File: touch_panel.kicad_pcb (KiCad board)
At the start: 2 copper layers, 50 x 50 mm, 46 parts, among them J1 2x4 SMD 2.0 MM, J2 2x4 Regular, Q1 MMBT2222, Q2 MMBT2222, Q3 MMBT2222, Q4 MMBT2222, Q5 MMBT2222, Q6 MMBT2222, SW1 Reset Switch, U1 TTP223_1, U2 TTP223_2, U3 TTP223_3, U4 ESP-12E

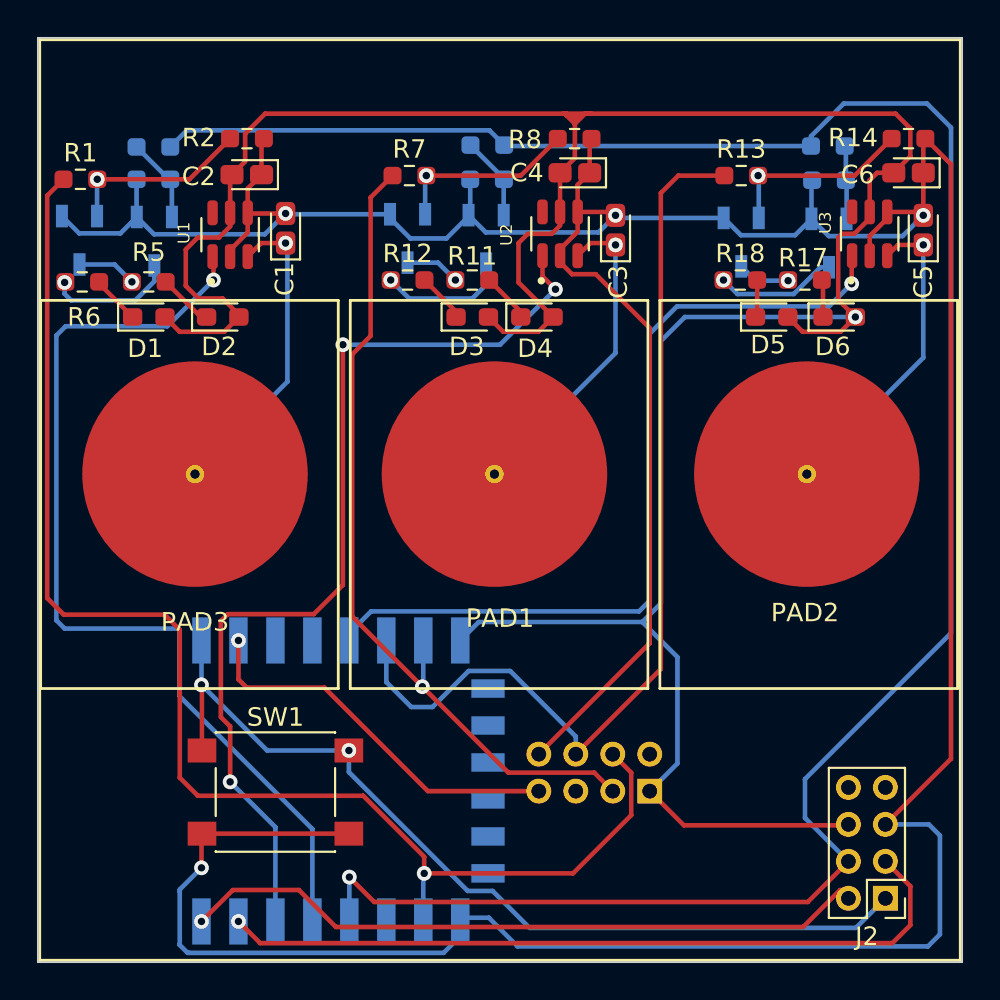
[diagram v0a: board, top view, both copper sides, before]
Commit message: Board finalized for printing
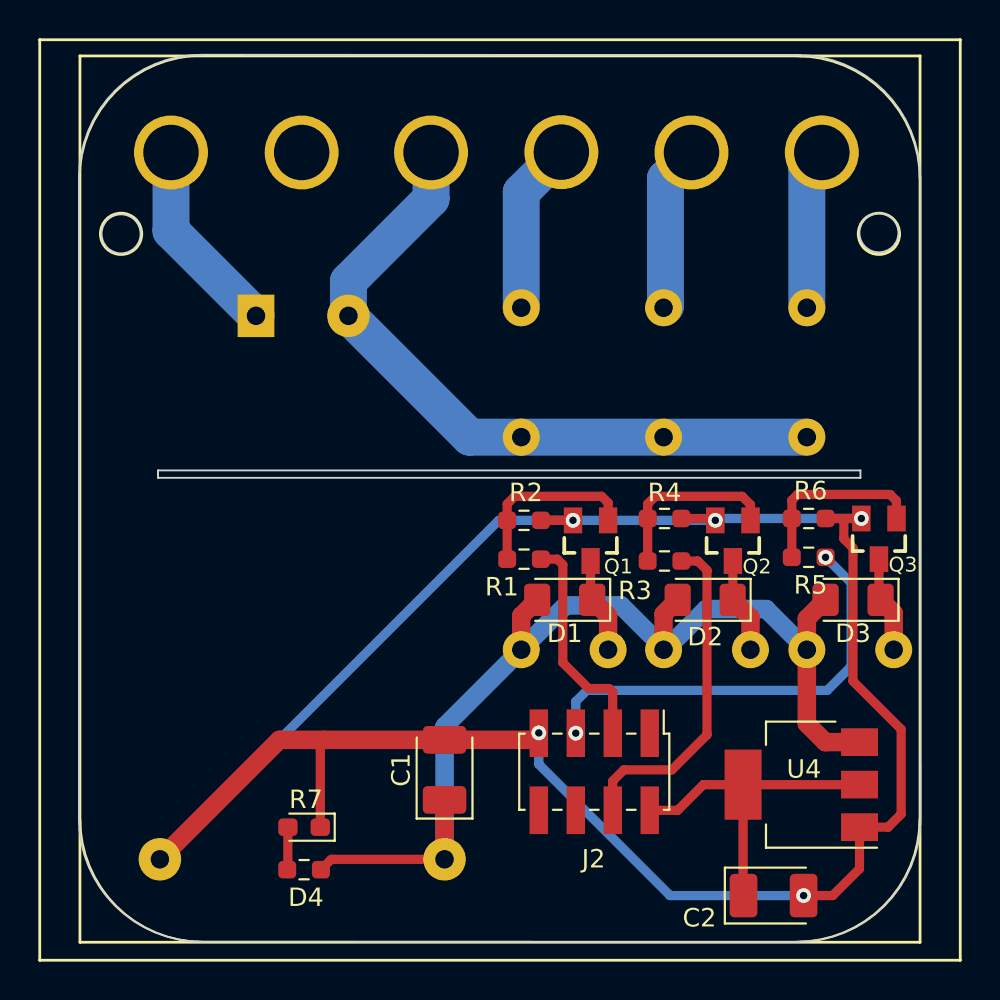
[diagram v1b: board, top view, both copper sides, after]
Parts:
- removed C3, C5: 0-50 pF (30 pF), Capacitor_Tantalum_SMD:CP_EIA-1608-10_AVX-L_Pad1.25x1.05mm_HandSolder
- removed C4, C6: 100nF, Capacitor_Tantalum_SMD:CP_EIA-1608-10_AVX-L_Pad1.25x1.05mm_HandSolder
- removed D5: BLUE, LED_SMD:LED_0603_1608Metric_Pad1.05x0.95mm_HandSolder
- removed D6: WHITE, LED_SMD:LED_0603_1608Metric_Pad1.05x0.95mm_HandSolder
- removed PAD1: Sense pad 1, Connector:senspad
- removed PAD2: Sense pad 2, Connector:senspad
- removed PAD3: Sense pad 3, Connector:senspad
- removed Q4, Q5, Q6: MMBT2222, Package_TO_SOT_SMD:TSOT-23
- removed R10, R14, R16, R8: 10K, Resistor_SMD:R_0603_1608Metric_Pad0.98x0.95mm_HandSolder
- removed R11, R12, R17, R18: 10R, Resistor_SMD:R_0603_1608Metric_Pad0.98x0.95mm_HandSolder
- removed R13, R15, R9: 1K, Resistor_SMD:R_0603_1608Metric_Pad0.98x0.95mm_HandSolder
- removed SW1: Reset Switch, Button_Switch_SMD:SW_Push_1P1T_NO_6x6mm_H9.5mm
- added PS1: HLK-PM01, Converter_ACDC:Converter_ACDC_HiLink_HLK-PMxx, B.Cu at (119.3, 94.4)
- C1: value 0-50 pF (30 pF) -> 22uF; footprint Capacitor_Tantalum_SMD:CP_EIA-1608-10_AVX-L_Pad1.25x1.05mm_HandSolder -> Capacitor_Tantalum_SMD:CP_EIA-3528-12_Kemet-T_Pad1.50x2.35mm_HandSolder
- C2: value 100nF -> 22uF; footprint Capacitor_Tantalum_SMD:CP_EIA-1608-10_AVX-L_Pad1.25x1.05mm_HandSolder -> Capacitor_Tantalum_SMD:CP_EIA-3528-12_Kemet-T_Pad1.50x2.35mm_HandSolder
- D1, D3: value BLUE -> DIODE; footprint LED_SMD:LED_0603_1608Metric_Pad1.05x0.95mm_HandSolder -> Diode_SMD:D_1206_3216Metric_Pad1.42x1.75mm_HandSolder
- D2: value WHITE -> DIODE; footprint LED_SMD:LED_0603_1608Metric_Pad1.05x0.95mm_HandSolder -> Diode_SMD:D_1206_3216Metric_Pad1.42x1.75mm_HandSolder
- D4: value WHITE -> RED
- J1: value 2x4 SMD 2.0 MM -> Screw_Terminal_01x06; footprint Connector_PinHeader_2.00mm:PinHeader_2x04_P2.00mm_Vertical -> Converter_ACDC:touch-relay
- J2: value 2x4 Regular -> 2x4 SMD 2.0 MM; footprint Connector_PinHeader_2.00mm:PinHeader_2x04_P2.00mm_Vertical -> Connector_PinHeader_2.00mm:PinHeader_2x04_P2.00mm_Vertical_SMD
- Q1, Q2, Q3: value MMBT2222 -> MMBT2222*; footprint Package_TO_SOT_SMD:TSOT-23 -> MMBT:SOT23-BEC; moved to F.Cu
- R3, R4: moved to F.Cu
- R5: value 10R -> 1K
- R6: value 10R -> 10K
- R7: value 1K -> 2K
- U1: value TTP223_1 -> c0942; footprint ttp223:SOT95P285X126-6N -> Relay_THT:c0942
- U2: value TTP223_2 -> c0942; footprint ttp223:SOT95P285X126-6N -> Relay_THT:c0942
- U3: value TTP223_3 -> c0942; footprint ttp223:SOT95P285X126-6N -> Relay_THT:c0942
- U4: value ESP-12E -> AMS1117-3.3; footprint RF_Module:ESP-12E -> Package_TO_SOT_SMD:SOT-223-3_TabPin2; moved to F.Cu
- moved C2 48.3 mm to (147.3, 125.8), turned to 0 degrees
- moved J1 43.2 mm to (114.7, 85.6)
- moved R6 41.3 mm to (149.2, 105.4), turned to 180 degrees
- moved R5 38.7 mm to (149.2, 107.5)
- moved R7 38.0 mm to (121.9, 124.4)
- moved R3 35.6 mm to (141.4, 107.7), turned to 0 degrees
- moved Q2 35.2 mm to (145.1, 106.6), turned to 180 degrees
- moved R4 33.2 mm to (141.4, 105.4), turned to 180 degrees
- moved Q1 32.1 mm to (137.4, 106.6), turned to 180 degrees
- moved R1 31.6 mm to (133.8, 107.6)
- moved C1 30.5 mm to (129.5, 119.0)
- moved D4 30.3 mm to (121.9, 122.1), turned to 180 degrees
- moved D2 30.3 mm to (143.6, 109.8), turned to 180 degrees
- moved Q3 30.2 mm to (153.0, 106.5), turned to 180 degrees
- moved U4 29.0 mm to (148.8, 119.8), turned to 180 degrees
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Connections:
- C1 pad 1: Net-(C1-Pad1) -> +5V
- C2 pad 1: GND -> +3V3
- C2 pad 2: +3V3 -> GND
- D1 pad 2: +3V3 -> +5V
- D2 pad 2: +3V3 -> +5V
- D3 pad 2: +3V3 -> +5V
- D4 pad 1: Net-(D4-Pad1) -> GND
- D4 pad 2: +3V3 -> Net-(D4-Pad2)
- J1 pad 1: +3V3 -> (no net)
- J1 pad 2: unconnected-(J1-Pad2) -> Neutral
- J1 pad 3: Relay 2 -> Phase
- J1 pad 4: Relay 1 -> Load 1
- J1 pad 5: unconnected-(J1-Pad5) -> Load 2
- J1 pad 6: Relay 3 -> Load 3
- J2 pad 1: RST -> +3V3
- J2 pad 2: TX -> (no net)
- J2 pad 3: RX -> Relay 2
- J2 pad 4: BLUELED -> Relay 1
- J2 pad 5: GND -> (no net)
- J2 pad 6: +3V3 -> Relay 3
- J2 pad 7: (no net) -> TEMP
- J2 pad 8: (no net) -> GND
- R1 pad 1: Relay 1 -> Net-(Q1-PadB)
- R1 pad 2: Net-(Q1-Pad2) -> Relay 1
- R2 pad 2: Net-(Q1-Pad2) -> Net-(Q1-PadB)
- R3 pad 1: BLUELED -> Net-(Q2-PadB)
- R3 pad 2: Net-(Q2-Pad2) -> Relay 2
- R4 pad 2: Net-(Q2-Pad2) -> Net-(Q2-PadB)
- R5 pad 1: Net-(Q1-Pad3) -> Net-(Q3-PadB)
- R5 pad 2: Net-(D2-Pad1) -> Relay 3
- R6 pad 1: Net-(Q2-Pad3) -> GND
- R6 pad 2: Net-(D1-Pad1) -> Net-(Q3-PadB)
- R7 pad 1: Relay 2 -> Net-(D4-Pad2)
- R7 pad 2: Net-(Q3-Pad2) -> +5V
- U1 pad 1: Touch 1 -> Load 1
- U1 pad 2: GND -> Phase
- U1 pad 3: Net-(C1-Pad1) -> +5V
- U1 pad 4: GND -> Net-(D1-Pad1)
- U2 pad 1: Touch 2 -> Load 2
- U2 pad 2: GND -> Phase
- U2 pad 3: Net-(C3-Pad1) -> +5V
- U2 pad 4: GND -> Net-(D2-Pad1)
- U3 pad 1: Touch 3 -> Load 3
- U3 pad 2: GND -> Phase
- U3 pad 3: Net-(C5-Pad1) -> +5V
- U3 pad 4: GND -> Net-(D3-Pad1)
- U4 pad 1: RST -> GND
- U4 pad 2: TEMP -> +3V3
- U4 pad 3: +3V3 -> +5V
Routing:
- net +3V3: track 152.3 -> 17.9 mm, vias 1 -> 0
- net BLUELED: track 118.8 -> 0.00 mm, vias 1 -> 0
- net GND: track 223.3 -> 124.3 mm, vias 4 -> 5
- net Relay 1: track 73.6 -> 13.8 mm, vias 1 -> 0
- net +5V: track 0.00 -> 58.9 mm
- net Touch 2: track 52.7 -> 0.00 mm, vias 3 -> 0
- net Touch 1: track 52.1 -> 0.00 mm, vias 1 -> 0
- net RST: track 49.8 -> 0.00 mm, vias 2 -> 0
- net Touch 3: track 46.1 -> 0.00 mm, vias 1 -> 0
- net RX: track 41.2 -> 0.00 mm, vias 1 -> 0
- net Phase: track 0.00 -> 38.2 mm
- net TX: track 37.5 -> 0.00 mm, vias 1 -> 0
- net Relay 3: track 52.4 -> 23.9 mm, vias 0 -> 2
- net Relay 2: track 45.3 -> 19.8 mm, vias 1 -> 0
- net TEMP: track 20.9 -> 0.00 mm, vias 1 -> 0
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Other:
- board size 50 x 50 mm -> 45.5 x 48 mm
